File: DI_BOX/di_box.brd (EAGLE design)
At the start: 59.4 x 29.2 mm, 10 parts, among them Q1 2N5950, X1 MC3FAH-0

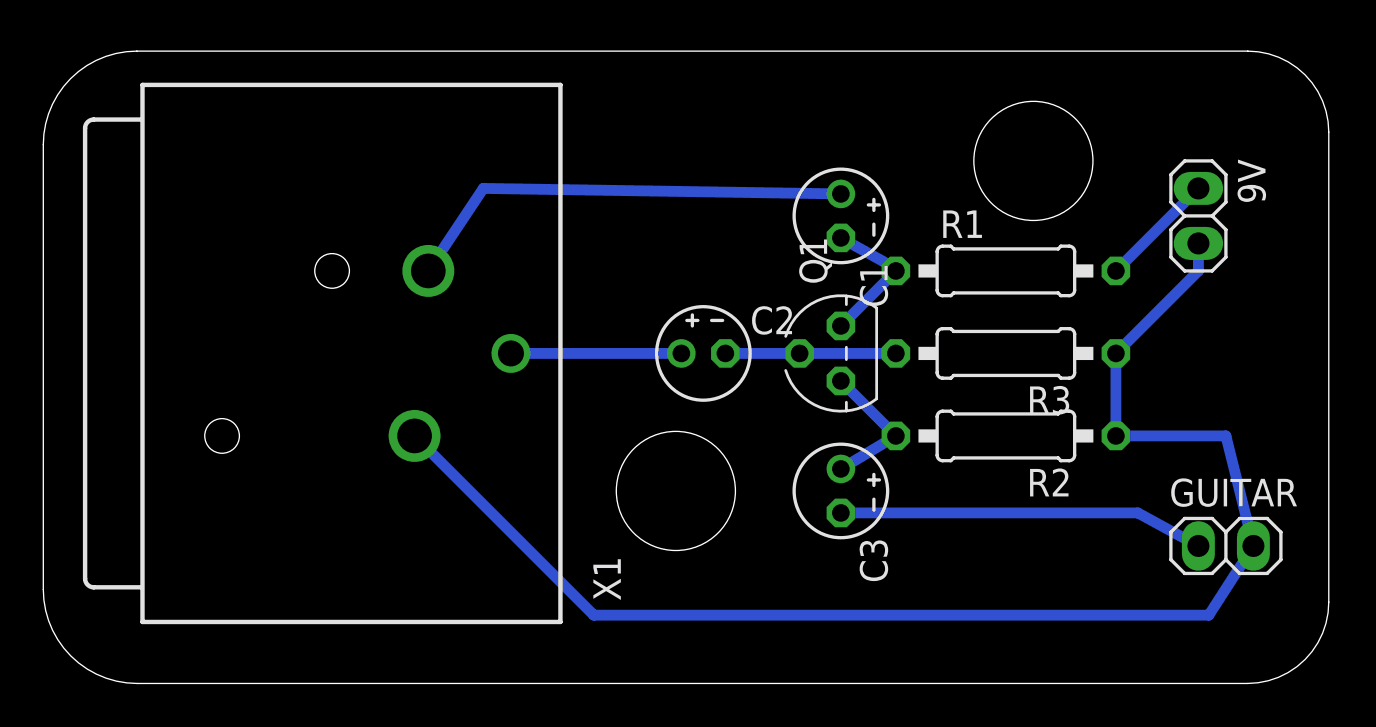
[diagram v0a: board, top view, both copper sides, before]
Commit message: updated schematic
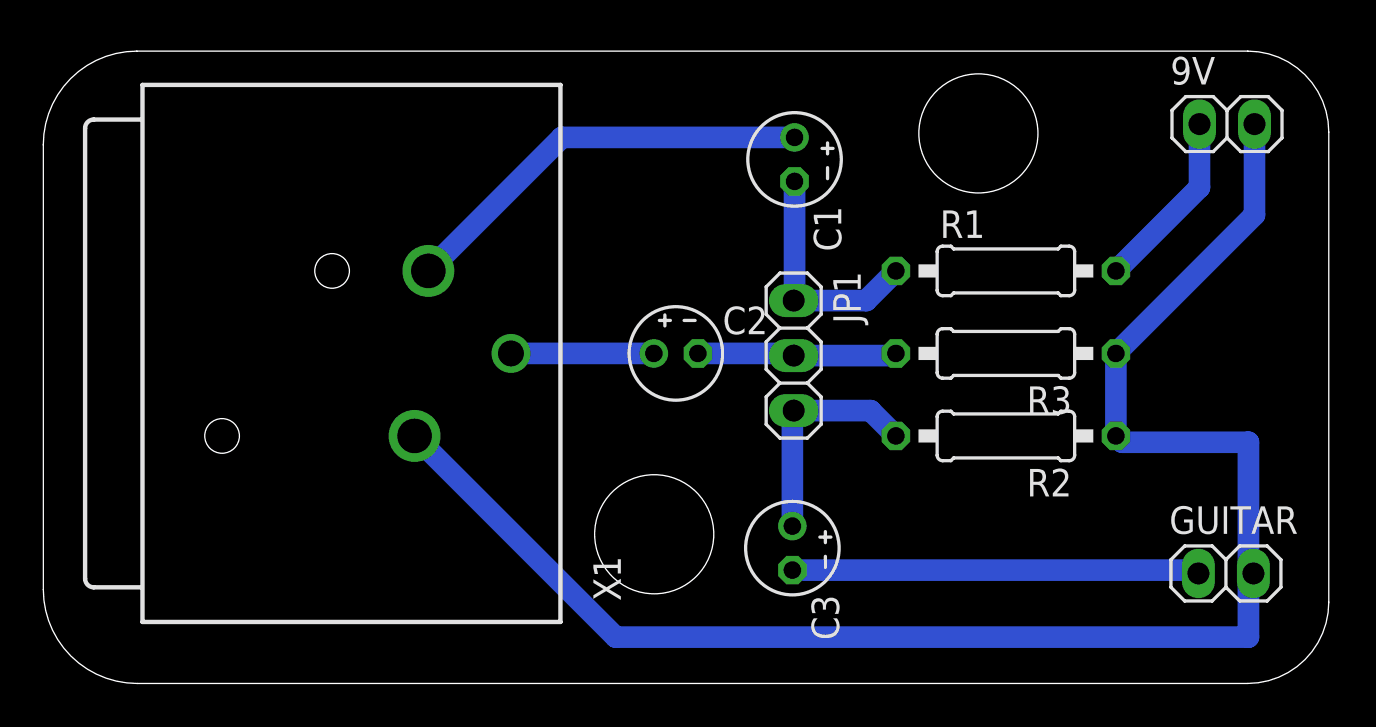
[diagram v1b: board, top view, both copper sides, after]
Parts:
- removed Q1: 2N5950, transistor-fet:TO-92
- added JP1: (no value), pinhead:1X03
- moved 9V 4.44 mm to (61.0, 48.7), turned to 0 degrees
- moved C3 3.46 mm to (40.9, 29.1)
- moved C1 3.38 mm to (41.0, 47.1)
- moved GUITAR 1.27 mm to (61.0, 27.9)
- moved C2 1.27 mm to (35.6, 38.1)
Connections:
- net N$1: now also JP1.3; no longer Q1.1
- net N$2: now also JP1.1; no longer Q1.3
- net N$4: now also JP1.2; no longer Q1.2
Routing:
- net N$3: track 64.7 -> 75.3 mm
- net N$2: track 6.57 -> 11.1 mm
- net N$1: track 6.55 -> 10.6 mm
- net N$6: track 5.39 -> 8.38 mm
- net N$5: track 16.9 -> 18.9 mm
- net N$8: track 21.1 -> 19.5 mm
- net N$4: track 7.87 -> 9.23 mm
- net N$7: track 7.87 -> 6.60 mm
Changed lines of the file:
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@@
 <setting verticaltext="up"/>
 </settings>
-<grid distance="50" unitdist="mil" unit="mm" style="lines" multiple="1" display="no" altdistance="5" altunitdist="mil" altunit="mil"/>
+<grid distance="1" unitdist="mm" unit="mm" style="lines" multiple="1" display="no" altdistance="5" altunitdist="mil" altunit="mil"/>
 <layers>
 <layer number="1" name="Top" color="4" fill="1" visible="yes" active="yes"/>
@@
 <layer number="47" name="Measures" color="7" fill="1" visible="no" active="yes"/>
 <layer number="48" name="Document" color="7" fill="1" visible="yes" active="yes"/>
-<layer number="49" name="Reference" color="7" fill="1" visible="yes" active="yes"/>
+<layer number="49" name="Reference" color="13" fill="1" visible="yes" active="yes"/>
 <layer number="50" name="dxf" color="7" fill="1" visible="no" active="no"/>
 <layer number="51" name="tDocu" color="7" fill="1" visible="yes" active="yes"/>
@@
 <wire x1="61.970921875" y1="52.06" x2="10.668959375" y2="52.06" width="0" layer="20"/>
 <wire x1="10.668959375" y1="52.06" x2="6.35" y2="47.741040625" width="0" layer="20" curve="90"/>
-<hole x="35.56" y="31.75" drill="5.5"/>
-<hole x="52.07" y="46.99" drill="5.5"/>
+<hole x="34.56" y="29.75" drill="5.5"/>
+<hole x="49.53" y="48.26" drill="5.5"/>
+<wire x1="43" y1="42" x2="43" y2="34" width="0.2" layer="49"/>
+<wire x1="43" y1="34" x2="43" y2="42" width="0.2" layer="49" curve="-180"/>
 </plain>
 <attributes>
@@
 </autorouter>
 <elements>
-<element name="9V" library="pinhead" library_urn="urn:adsk.eagle:library:325" package="1X02" package3d_urn="urn:adsk.eagle:package:22435/2" value="" x="59.69" y="44.45" rot="R270"/>
-<element name="C1" library="rcl" library_urn="urn:adsk.eagle:library:334" package="E2-4" package3d_urn="urn:adsk.eagle:package:23347/1" value="10 uF" x="43.18" y="44.45" rot="R270">
-<attribute name="SPICEPREFIX" value="C" x="43.18" y="44.45" size="1.778" layer="27" rot="R270" display="off"/>
-</element>
-<element name="C2" library="rcl" library_urn="urn:adsk.eagle:library:334" package="E2-4" package3d_urn="urn:adsk.eagle:package:23347/1" value="10 uF" x="36.83" y="38.1">
-<attribute name="SPICEPREFIX" value="C" x="36.83" y="38.1" size="1.778" layer="27" display="off"/>
-</element>
-<element name="C3" library="rcl" library_urn="urn:adsk.eagle:library:334" package="E2-4" package3d_urn="urn:adsk.eagle:package:23347/1" value="10 uF" x="43.18" y="31.75" rot="R270">
-<attribute name="SPICEPREFIX" value="C" x="43.18" y="31.75" size="1.778" layer="27" rot="R270" display="off"/>
-</element>
-<element name="GUITAR" library="pinhead" library_urn="urn:adsk.eagle:library:325" package="1X02" package3d_urn="urn:adsk.eagle:package:22435/2" value="" x="60.96" y="29.21"/>
-<element name="Q1" library="transistor-fet" library_urn="urn:adsk.eagle:library:396" package="TO-92" package3d_urn="urn:adsk.eagle:package:28535/2" value="2N5950" x="43.18" y="38.1" rot="R90"/>
+<element name="9V" library="pinhead" library_urn="urn:adsk.eagle:library:325" package="1X02" package3d_urn="urn:adsk.eagle:package:22435/2" value="" x="61.01" y="48.69"/>
+<element name="C1" library="rcl" library_urn="urn:adsk.eagle:library:334" package="E2-4" package3d_urn="urn:adsk.eagle:package:23347/1" value="10 uF" x="41.04" y="47.06" rot="R270">
+<attribute name="SPICEPREFIX" value="C" x="41.04" y="47.06" size="1.778" layer="27" rot="R270" display="off"/>
+</element>
+<element name="C2" library="rcl" library_urn="urn:adsk.eagle:library:334" package="E2-4" package3d_urn="urn:adsk.eagle:package:23347/1" value="10 uF" x="35.56" y="38.1">
+<attribute name="SPICEPREFIX" value="C" x="35.56" y="38.1" size="1.778" layer="27" display="off"/>
+</element>
+<element name="C3" library="rcl" library_urn="urn:adsk.eagle:library:334" package="E2-4" package3d_urn="urn:adsk.eagle:package:23347/1" value="10 uF" x="40.94" y="29.11" rot="R270">
+<attribute name="SPICEPREFIX" value="C" x="40.94" y="29.11" size="1.778" layer="27" rot="R270" display="off"/>
+</element>
+<element name="GUITAR" library="pinhead" library_urn="urn:adsk.eagle:library:325" package="1X02" package3d_urn="urn:adsk.eagle:package:22435/2" value="" x="60.96" y="27.94"/>
 <element name="R1" library="rcl" library_urn="urn:adsk.eagle:library:334" package="0207/10" package3d_urn="urn:adsk.eagle:package:23491/1" value="6.8K" x="50.8" y="41.91">
 <attribute name="SPICEPREFIX" value="R" x="50.8" y="41.91" size="1.778" layer="27" display="off"/>
@@
 <attribute name="OC_NEWARK" value="unknown" x="24.13" y="38.1" size="1.778" layer="27" rot="R90" display="off"/>
 </element>
+<element name="JP1" library="pinhead" library_urn="urn:adsk.eagle:library:325" package="1X03" package3d_urn="urn:adsk.eagle:package:22458/2" value="" x="41" y="38" rot="R270"/>
 </elements>
 <signals>
@@
 <contactref element="C3" pad="+"/>
 <contactref element="R2" pad="2"/>
-<contactref element="Q1" pad="1"/>
-<wire x1="43.18" y1="36.83" x2="45.72" y2="34.29" width="0.5" layer="16"/>
-<wire x1="45.72" y1="34.29" x2="43.18" y2="32.766" width="0.5" layer="16"/>
+<contactref element="JP1" pad="3"/>
+<wire x1="45.72" y1="34.29" x2="44.55" y2="35.46" width="1" layer="16"/>
+<wire x1="44.55" y1="35.46" x2="41" y2="35.46" width="1" layer="16"/>
+<wire x1="40.94" y1="30.126" x2="40.94" y2="35.4" width="1" layer="16"/>
+<wire x1="40.94" y1="35.4" x2="41" y2="35.46" width="1" layer="16"/>
 </signal>
 <signal name="N$3">
@@
 <contactref element="9V" pad="2"/>
 <contactref element="GUITAR" pad="2"/>
-<wire x1="55.88" y1="34.29" x2="55.88" y2="38.1" width="0.5" layer="16"/>
-<wire x1="55.88" y1="38.1" x2="59.69" y2="41.91" width="0.5" layer="16"/>
-<wire x1="59.69" y1="41.91" x2="59.69" y2="43.18" width="0.5" layer="16"/>
-<wire x1="23.495" y1="34.29" x2="31.7714" y2="26.0136" width="0.5" layer="16"/>
-<wire x1="31.7714" y1="26.0136" x2="60.1723125" y2="26.0136" width="0.5" layer="16"/>
-<wire x1="55.88" y1="34.29" x2="60.96" y2="34.29" width="0.5" layer="16"/>
-<wire x1="60.96" y1="34.29" x2="62.23" y2="29.21" width="0.5" layer="16"/>
-<wire x1="62.23" y1="29.21" x2="60.1723125" y2="26.0136" width="0.5" layer="16"/>
+<wire x1="23.495" y1="34.29" x2="32.785" y2="25" width="1" layer="16"/>
+<wire x1="32.785" y1="25" x2="62" y2="25" width="1" layer="16"/>
+<wire x1="62" y1="25" x2="62" y2="27.71" width="1" layer="16"/>
+<wire x1="62" y1="27.71" x2="62.23" y2="27.94" width="1" layer="16"/>
+<wire x1="62.23" y1="27.94" x2="62" y2="28.17" width="1" layer="16"/>
+<wire x1="55.88" y1="34.29" x2="55.88" y2="38.1" width="1" layer="16"/>
+<wire x1="55.88" y1="34.29" x2="56.17" y2="34" width="1" layer="16"/>
+<wire x1="56.17" y1="34" x2="62" y2="34" width="1" layer="16"/>
+<wire x1="62" y1="34" x2="62" y2="27.71" width="1" layer="16"/>
+<wire x1="55.88" y1="38.1" x2="62.28" y2="44.5" width="1" layer="16"/>
+<wire x1="62.28" y1="44.5" x2="62.28" y2="48.69" width="1" layer="16"/>
 </signal>
 <signal name="N$4">
-<contactref element="Q1" pad="2"/>
 <contactref element="R3" pad="2"/>
 <contactref element="C2" pad="-"/>
-<wire x1="37.846" y1="38.1" x2="41.275" y2="38.1" width="0.5" layer="16"/>
-<wire x1="41.275" y1="38.1" x2="45.72" y2="38.1" width="0.5" layer="16"/>
+<contactref element="JP1" pad="2"/>
+<wire x1="36.576" y1="38.1" x2="40.9" y2="38.1" width="1" layer="16"/>
+<wire x1="40.9" y1="38.1" x2="41" y2="38" width="1" layer="16"/>
+<wire x1="41" y1="38" x2="45.62" y2="38" width="1" layer="16"/>
+<wire x1="45.62" y1="38" x2="45.72" y2="38.1" width="1" layer="16"/>
 </signal>
 <signal name="N$2">
-<contactref element="Q1" pad="3"/>
 <contactref element="R1" pad="1"/>
 <contactref element="C1" pad="-"/>
-<wire x1="43.18" y1="43.434" x2="45.466" y2="42.164" width="0.5" layer="16"/>
-<wire x1="45.466" y1="42.164" x2="45.72" y2="41.91" width="0.5" layer="16"/>
-<wire x1="43.18" y1="39.37" x2="45.72" y2="41.91" width="0.5" layer="16"/>
+<wire x1="41.04" y1="45.79" x2="41.04" y2="46.044" width="1" layer="16"/>
+<contactref element="JP1" pad="1"/>
+<wire x1="41" y1="40.54" x2="44.35" y2="40.54" width="1" layer="16"/>
+<wire x1="44.35" y1="40.54" x2="45.72" y2="41.91" width="1" layer="16"/>
+<wire x1="41.04" y1="46.044" x2="41.04" y2="40.58" width="1" layer="16"/>
+<wire x1="41.04" y1="40.58" x2="41" y2="40.54" width="1" layer="16"/>
 </signal>
 <signal name="N$6">
 <contactref element="R1" pad="2"/>
 <contactref element="9V" pad="1"/>
-<wire x1="55.88" y1="41.91" x2="59.69" y2="45.72" width="0.5" layer="16"/>
+<wire x1="55.88" y1="41.91" x2="59.74" y2="45.77" width="1" layer="16"/>
+<wire x1="59.74" y1="45.77" x2="59.74" y2="48.69" width="1" layer="16"/>
 </signal>
 <signal name="N$7">
 <contactref element="C2" pad="+"/>
 <contactref element="X1" pad="3"/>
-<wire x1="27.945" y1="38.1" x2="35.814" y2="38.1" width="0.5" layer="16"/>
+<wire x1="27.945" y1="38.1" x2="34.544" y2="38.1" width="1" layer="16"/>
 </signal>
 <signal name="N$8">
 <contactref element="C1" pad="+"/>
 <contactref element="X1" pad="2"/>
-<wire x1="43.18" y1="45.466" x2="26.67" y2="45.72" width="0.5" layer="16"/>
-<wire x1="26.67" y1="45.72" x2="24.13" y2="41.91" width="0.5" layer="16"/>
+<wire x1="24.13" y1="41.91" x2="30.296" y2="48.076" width="1" layer="16"/>
+<wire x1="30.296" y1="48.076" x2="41.04" y2="48.076" width="1" layer="16"/>
 </signal>
 <signal name="N$5">
 <contactref element="GUITAR" pad="1"/>
 <contactref element="C3" pad="-"/>
-<wire x1="43.18" y1="30.734" x2="56.896" y2="30.734" width="0.5" layer="16"/>
-<wire x1="56.896" y1="30.734" x2="59.69" y2="29.21" width="0.5" layer="16"/>
+<wire x1="59.436" y1="28.194" x2="59.69" y2="27.94" width="1" layer="16"/>
+<wire x1="40.94" y1="28.094" x2="59.336" y2="28.094" width="1" layer="16"/>
+<wire x1="59.336" y1="28.094" x2="59.436" y2="28.194" width="1" layer="16"/>
 </signal>
 </signals>
